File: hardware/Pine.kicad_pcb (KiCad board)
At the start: 2 copper layers, 45.7 x 58.4 mm, 46 parts, among them J1 USB Micro type-B, J2 01x06 Male conn, J3 Battery connector, Q1 p-channel MOSFET, Q2 NPN Transistor, SW1 Switch, SW2 Push button, U1 IR Receiver, U2 LDO, U3 Temperature sensor, U4 MCU

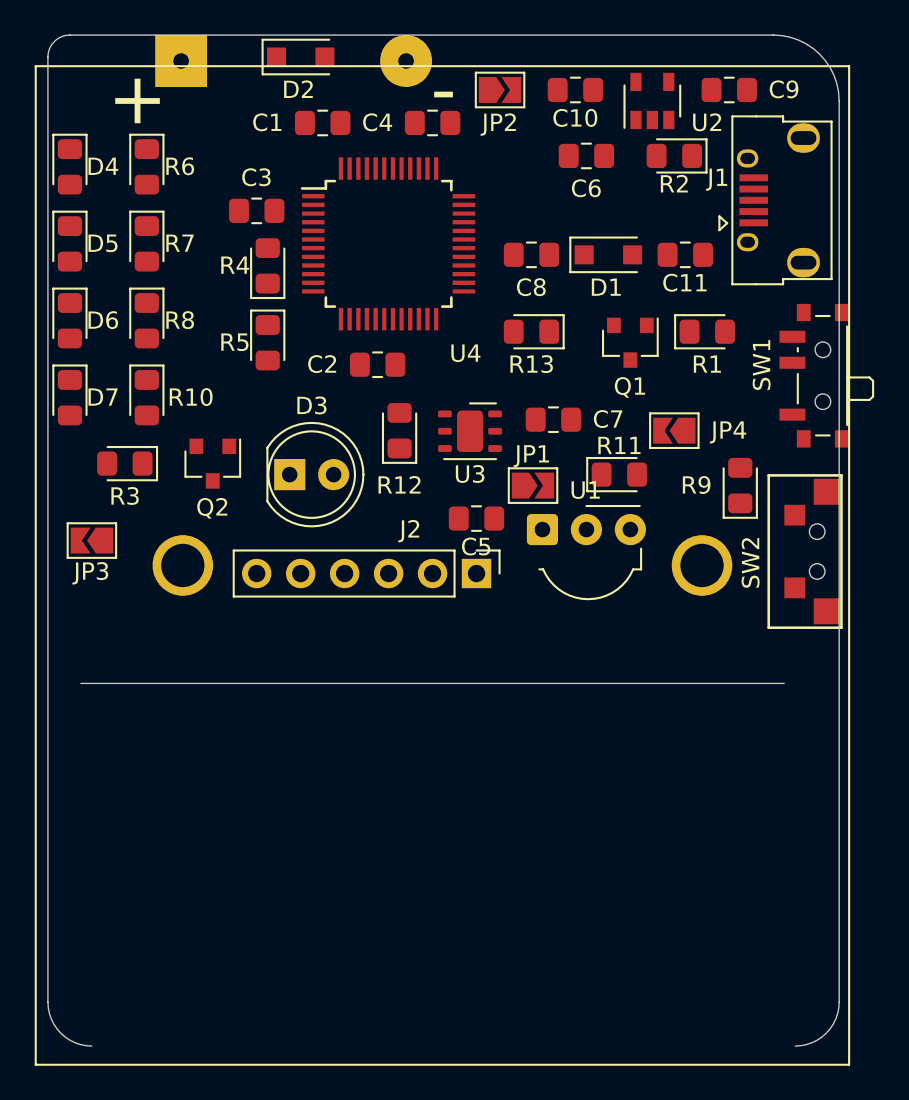
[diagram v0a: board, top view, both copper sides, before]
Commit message: feat: place components mechanically with silkscreen annotations
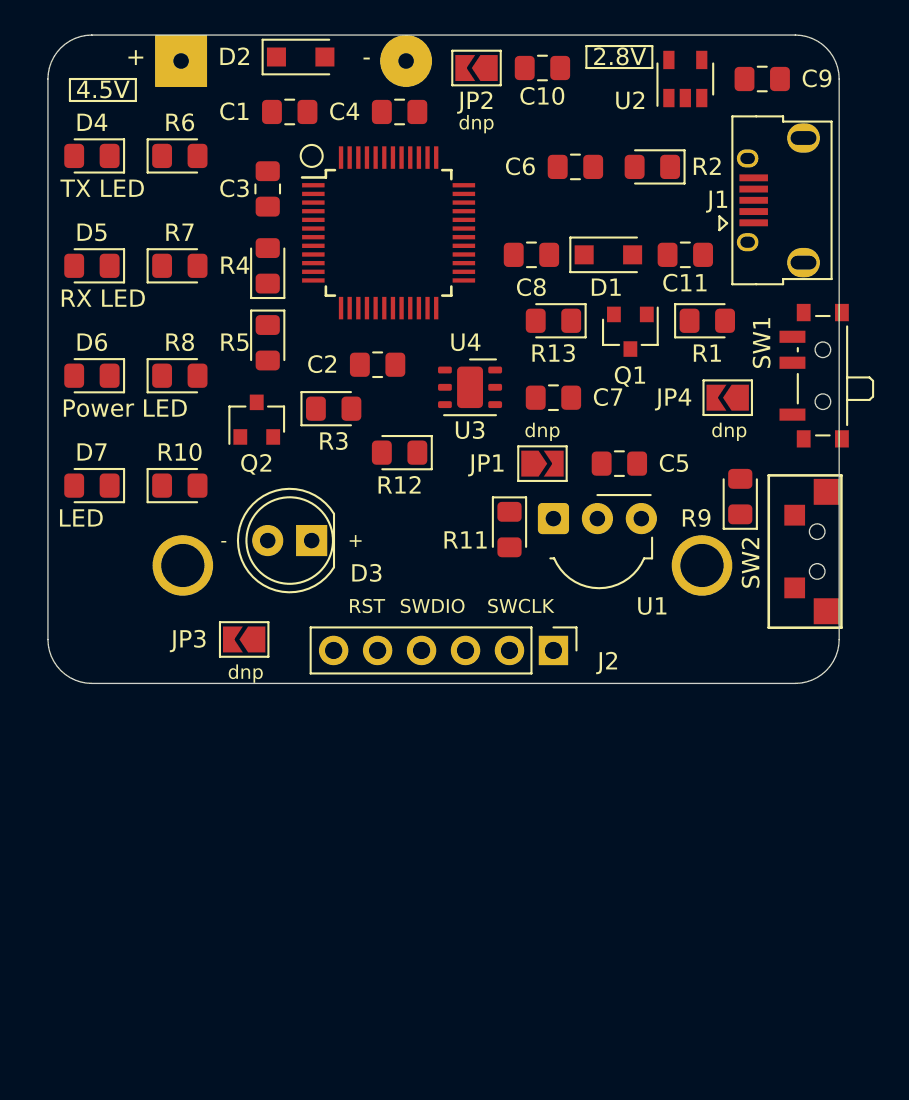
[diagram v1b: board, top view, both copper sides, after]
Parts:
- added REF**: OSHW-Logo2_9.8x8mm_SilkScreen, Symbol:OSHW-Logo2_9.8x8mm_SilkScreen, B.Cu at (175.9, 59.1)
- moved R3 12.5 mm to (169.5, 64.1), turned to 0 degrees
- moved JP3 10.5 mm to (164.4, 77.5)
- moved C5 8.84 mm to (186.1, 67.3)
- moved R11 7.10 mm to (179.7, 71.1), turned to 270 degrees
- moved J2 6.29 mm to (182.2, 78.1)
- moved R10 5.43 mm to (160.7, 68.6), turned to 0 degrees
- moved D7 5.24 mm to (155.6, 68.6), turned to 180 degrees
- moved D3 4.02 mm to (168.3, 71.8), turned to 180 degrees
- moved R8 3.70 mm to (160.7, 62.2), turned to 0 degrees
- moved JP4 3.63 mm to (192.3, 63.5)
- moved Q2 3.59 mm to (165.1, 64.8), turned to 90 degrees
- moved D6 3.42 mm to (155.6, 62.2), turned to 180 degrees
- moved U3 2.54 mm to (177.4, 62.9)
- moved R7 2.29 mm to (160.7, 55.9), turned to 0 degrees
- moved U2 2.29 mm to (189.9, 45.1)
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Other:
- board size 45.7 x 58.4 mm -> 45.7 x 37.5 mm
- board text added: "+"
- board text added: "-"
- board text added: "2.8V"
- board text added: "4.5V"
- board text added: "4.5V 3 AA"
- board text added: "D3"
- board text added: "Get started at hutscape.com/pine"
- board text added: "J1"
- board text added: "LED"
- board text added: "Pine@Hutscape V1.0 2019"
- board text added: "Power LED"
- board text added: "RST"
- board text added: "RX LED"
- board text added: "SW1"
- board text added: "SW2"
- board text added: "SWCLK"
- board text added: "SWDIO"
- board text added: "TX LED"
- board text added: "U1"
- board text added: "dnp"
